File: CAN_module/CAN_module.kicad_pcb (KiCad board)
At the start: 2 copper layers, 52 parts, among them IC1 SN65HVD233QDRQ1, J2 Barrel_Jack_Switch, J4 Conn_Coaxial, J5 Screw_Terminal_01x02, U1 PC817, U2 LM5164QDDATQ1, U3 Antena BT - 2450AT42E010B001E

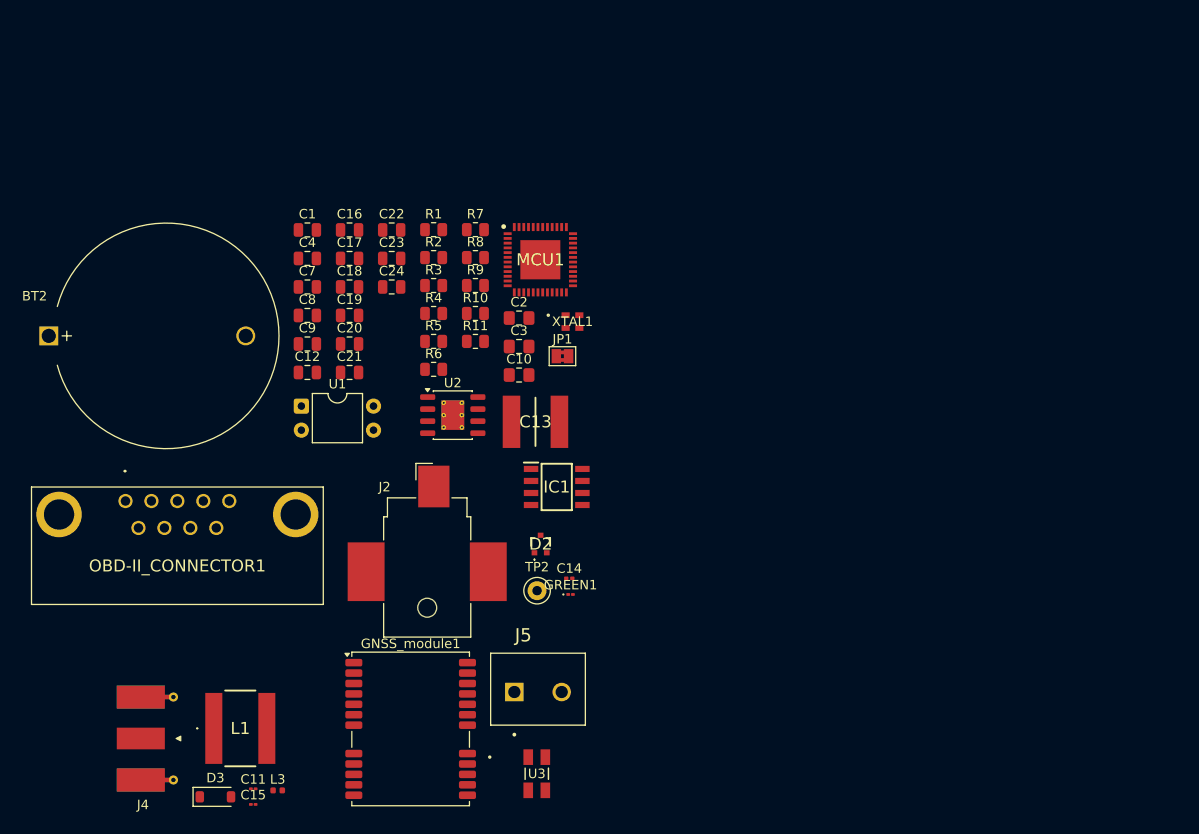
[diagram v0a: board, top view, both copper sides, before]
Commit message: Add files via upload
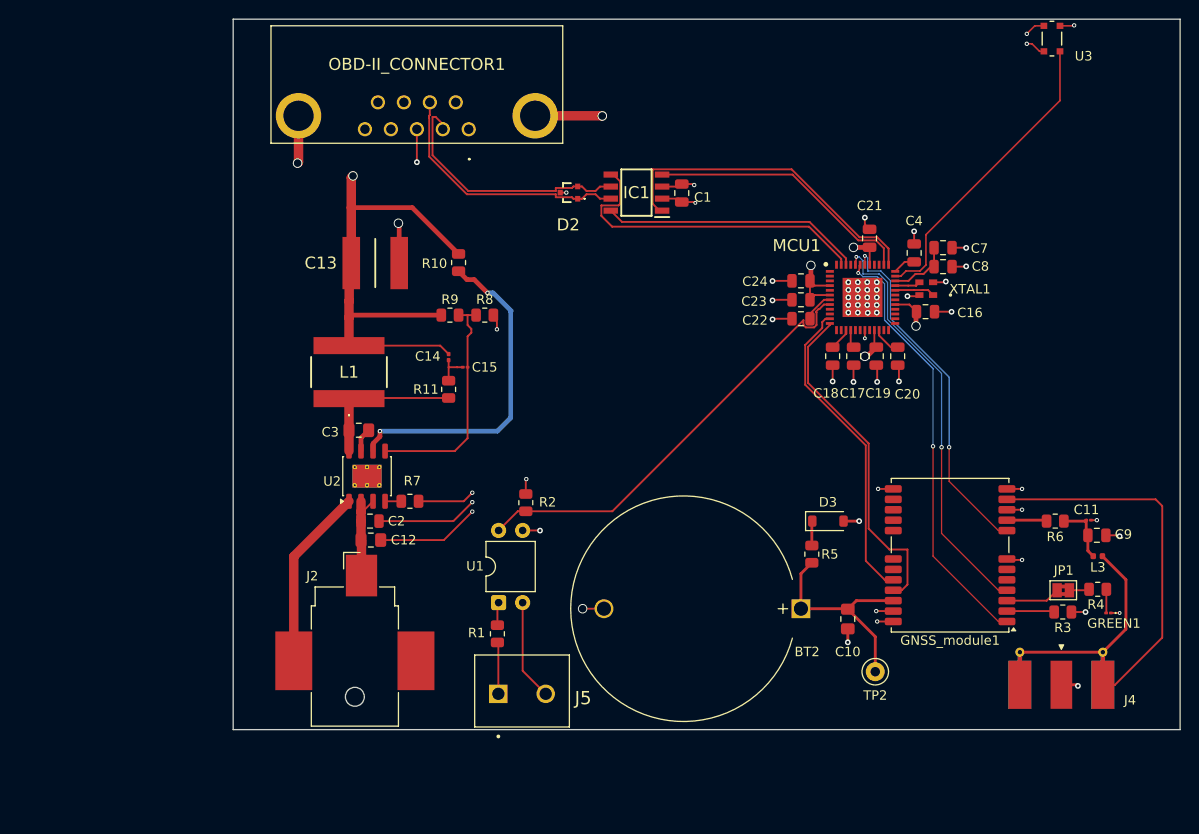
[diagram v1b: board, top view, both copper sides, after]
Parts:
- U3: value Antena BT - 2450AT42E010B001E -> Ant BT - 2450AT18D0100E; footprint Antyradar_footprints:2450AT42E010B_JOT -> Antyradar_footprints:2450AT18D0100E_JOT
- moved J4 95.8 mm to (200.4, 115.7), turned to 90 degrees
- moved U3 94.8 mm to (199.4, 49.2), turned to 180 degrees
- moved C11 92.7 mm to (203.3, 100.0), turned to 180 degrees
- moved L3 90.1 mm to (204.2, 103.8), turned to 180 degrees
- moved C9 85.8 mm to (204.1, 101.7), turned to 180 degrees
- moved BT2 84.5 mm to (172.9, 109.4), turned to 180 degrees
- moved R4 75.9 mm to (204.2, 107.3)
- moved R3 74.8 mm to (200.5, 109.8), turned to 180 degrees
- moved D3 70.9 mm to (175.7, 100.2)
- moved R6 67.6 mm to (199.7, 100.2), turned to 180 degrees
- moved C8 67.3 mm to (187.9, 73.3)
- moved C7 67.2 mm to (187.9, 71.3)
- moved C4 64.1 mm to (184.9, 71.8), turned to 90 degrees
- moved C16 61.4 mm to (186.1, 78.0)
- moved GNSS_module1 59.8 mm to (188.6, 103.8), turned to 180 degrees
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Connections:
- net Net-(D2-CATHODE_1) renamed /CAN_P
- net Net-(D2-CATHODE_2) renamed /CAN_N
- U3 pad 1: Net-(U3-FEEDING_POINT) -> /Antenna_BT
- U3 pad 2: unconnected-(U3-NC-Pad2) -> GND
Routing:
- net GND: track 0.00 -> 100.8 mm, vias 0 -> 59
- net +3.3V: track 0.00 -> 84.7 mm, vias 0 -> 11
- net /GPS_ANT: track 0.00 -> 59.9 mm
- net /AR_IN: track 0.00 -> 46.8 mm
- net /SB_GPS: track 0.00 -> 45.8 mm, vias 0 -> 2
- net /EXT_GPS: track 0.00 -> 44.4 mm, vias 0 -> 2
- net /RST_GPS: track 0.00 -> 37.6 mm, vias 0 -> 2
- net /GPS_RX: track 0.00 -> 35.7 mm
- net Net-(U2-PGOOD): track 0.00 -> 35.4 mm, vias 0 -> 2
- net /CAN0_TX: track 0.00 -> 35.0 mm
- net /LBK_CAN: track 0.00 -> 34.4 mm
- net /GPS_TX: track 0.00 -> 33.3 mm
- net /Antenna_BT: track 0.00 -> 32.2 mm
- net /CAN0_RX: track 0.00 -> 28.4 mm
- net /RS_CAN: track 0.00 -> 27.6 mm
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- added copper zone on In2.Cu, net +3.3V
- added copper zone on In1.Cu, net GND
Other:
- board outline added: 100 x 75 mm
- copper layers 2 -> 4
